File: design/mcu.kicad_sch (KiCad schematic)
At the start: 34 parts, among them J2 SWD_01X06, J3 DEBUG_SPI, U6 STM32H750VBTx, X1 ASTX-H11-25.000MHZ-T, X2 SIT8209AI-21-33S-100.000000X

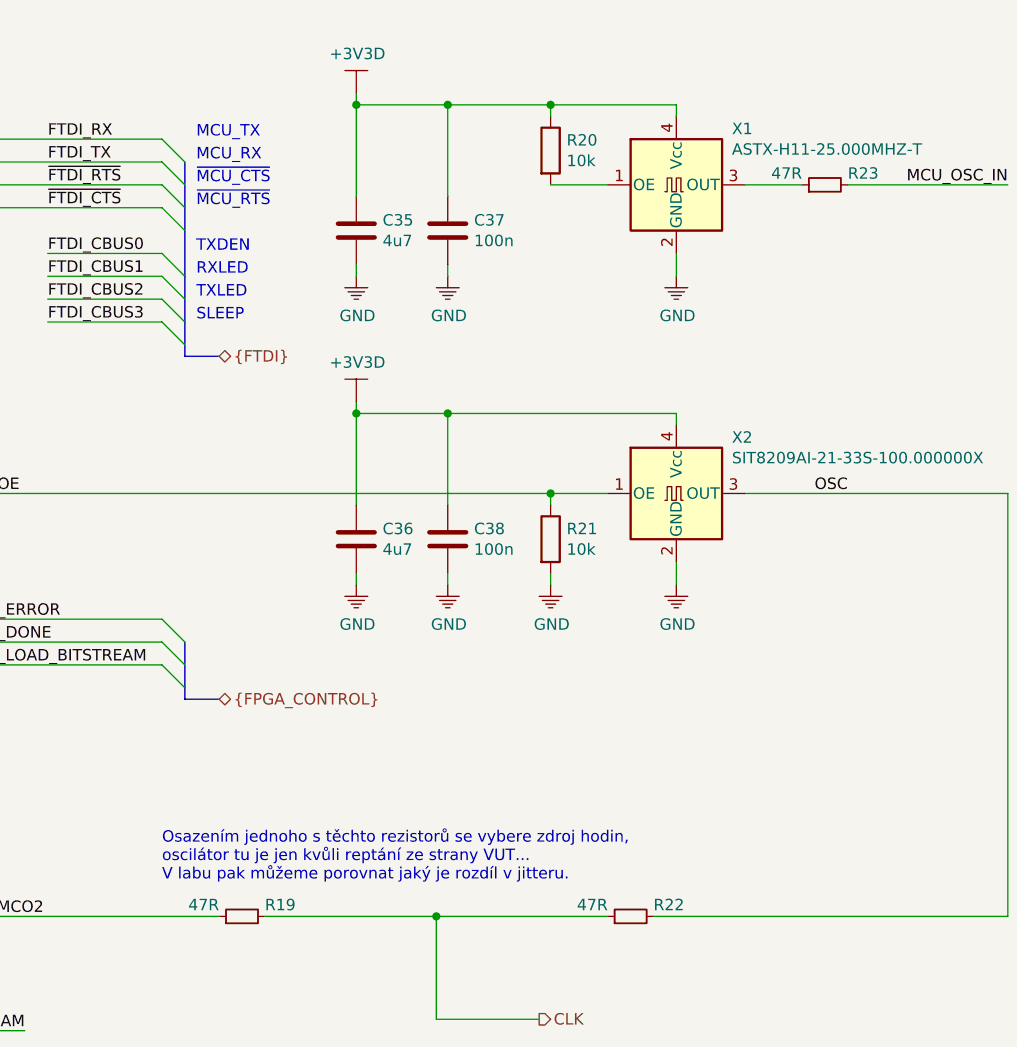
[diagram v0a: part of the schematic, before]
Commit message: Updated schematic
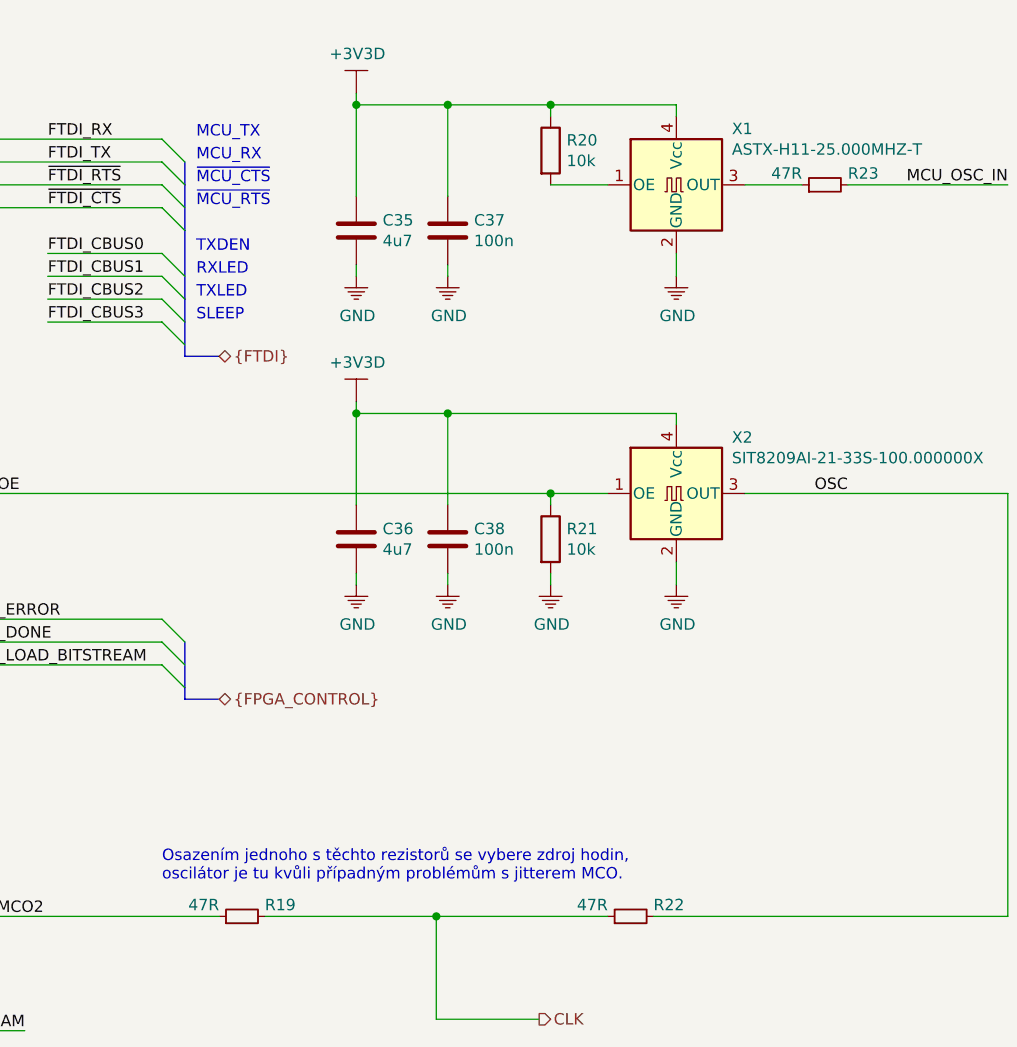
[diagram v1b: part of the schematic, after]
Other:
- note added: "Osazením jednoho s těchto rezistorů se vybere zdroj hodin, oscilátor je tu kvůli případným problémům s jitterem MCO."
- note removed: "Osazením jednoho s těchto rezistorů se vybere zdroj hodin, oscilátor tu je jen kvůli reptání ze strany VUT... V labu pak můžeme porovnat jaký je rozdíl v jitteru."
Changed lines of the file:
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@@
   (junction (at 236.22 25.4))
   (junction (at 262.89 26.67))
+  (no_connect (at 95.25 116.84))
+  (no_connect (at 140.97 48.26))
+  (no_connect (at 140.97 91.44))
+  (no_connect (at 95.25 152.4))
+  (no_connect (at 95.25 144.78))
+  (no_connect (at 140.97 96.52))
+  (no_connect (at 140.97 83.82))
+  (no_connect (at 140.97 58.42))
+  (no_connect (at 95.25 129.54))
+  (no_connect (at 140.97 93.98))
   (no_connect (at 140.97 43.18))
-  (no_connect (at 140.97 104.14))
+  (no_connect (at 95.25 132.08))
+  (no_connect (at 140.97 109.22))
+  (no_connect (at 140.97 134.62))
+  (no_connect (at 140.97 132.08))
+  (no_connect (at 140.97 129.54))
+  (no_connect (at 95.25 119.38))
+  (no_connect (at 140.97 119.38))
+  (no_connect (at 140.97 137.16))
+  (no_connect (at 140.97 101.6))
+  (no_connect (at 140.97 124.46))
+  (no_connect (at 95.25 137.16))
   (no_connect (at 140.97 149.86))
-  (no_connect (at 95.25 139.7))
+  (no_connect (at 140.97 45.72))
+  (no_connect (at 140.97 106.68))
+  (no_connect (at 140.97 53.34))
+  (no_connect (at 95.25 88.9))
+  (no_connect (at 95.25 109.22))
+  (no_connect (at 95.25 147.32))
+  (no_connect (at 140.97 76.2))
   (no_connect (at 95.25 99.06))
-  (no_connect (at 95.25 109.22))
-  (no_connect (at 140.97 134.62))
-  (no_connect (at 140.97 129.54))
+  (no_connect (at 140.97 50.8))
+  (no_connect (at 95.25 111.76))
+  (no_connect (at 95.25 76.2))
+  (no_connect (at 140.97 99.06))
   (no_connect (at 140.97 142.24))
   (no_connect (at 95.25 134.62))
+  (no_connect (at 95.25 104.14))
+  (no_connect (at 140.97 127))
   (no_connect (at 95.25 149.86))
-  (no_connect (at 140.97 93.98))
-  (no_connect (at 140.97 53.34))
-  (no_connect (at 140.97 137.16))
-  (no_connect (at 95.25 144.78))
-  (no_connect (at 140.97 76.2))
-  (no_connect (at 95.25 116.84))
-  (no_connect (at 140.97 91.44))
+  (no_connect (at 95.25 142.24))
+  (no_connect (at 95.25 83.82))
   (no_connect (at 140.97 38.1))
-  (no_connect (at 95.25 152.4))
-  (no_connect (at 95.25 119.38))
-  (no_connect (at 95.25 137.16))
-  (no_connect (at 140.97 99.06))
-  (no_connect (at 140.97 96.52))
-  (no_connect (at 140.97 124.46))
-  (no_connect (at 140.97 45.72))
-  (no_connect (at 140.97 132.08))
+  (no_connect (at 95.25 139.7))
+  (no_connect (at 140.97 157.48))
   (no_connect (at 95.25 81.28))
-  (no_connect (at 95.25 104.14))
-  (no_connect (at 95.25 83.82))
+  (no_connect (at 140.97 104.14))
+  (no_connect (at 140.97 144.78))
+  (no_connect (at 140.97 139.7))
+  (no_connect (at 140.97 162.56))
+  (no_connect (at 140.97 40.64))
+  (no_connect (at 95.25 114.3))
   (no_connect (at 140.97 55.88))
-  (no_connect (at 95.25 111.76))
-  (no_connect (at 140.97 127))
-  (no_connect (at 140.97 50.8))
-  (no_connect (at 140.97 157.48))
-  (no_connect (at 95.25 142.24))
-  (no_connect (at 95.25 76.2))
-  (no_connect (at 140.97 106.68))
-  (no_connect (at 140.97 48.26))
-  (no_connect (at 95.25 88.9))
-  (no_connect (at 140.97 40.64))
-  (no_connect (at 140.97 162.56))
-  (no_connect (at 140.97 109.22))
-  (no_connect (at 140.97 83.82))
-  (no_connect (at 95.25 147.32))
-  (no_connect (at 140.97 144.78))
-  (no_connect (at 140.97 101.6))
-  (no_connect (at 140.97 139.7))
-  (no_connect (at 95.25 114.3))
-  (no_connect (at 95.25 132.08))
-  (no_connect (at 140.97 119.38))
-  (no_connect (at 95.25 129.54))
-  (no_connect (at 140.97 58.42))
   (bus_entry (at 67.31 88.9) (size 2.54 -2.54))
   (bus_entry (at 67.31 93.98) (size 2.54 -2.54))
@@
   (bus (pts (xy 67.31 106.68) (xy 67.31 111.76)))
   (bus (pts (xy 67.31 111.76) (xy 67.31 113.03)))
-  (bus (pts (xy 182.88 63.5) (xy 182.88 68.58)))
-  (bus (pts (xy 182.88 68.58) (xy 182.88 76.2)))
-  (bus (pts (xy 182.88 76.2) (xy 182.88 81.28)))
+  (bus (pts (xy 182.88 63.5) (xy 182.88 66.04)))
+  (bus (pts (xy 182.88 66.04) (xy 182.88 71.12)))
+  (bus (pts (xy 182.88 71.12) (xy 182.88 78.74)))
+  (bus (pts (xy 182.88 78.74) (xy 182.88 81.28)))
   (bus (pts (xy 182.88 81.28) (xy 182.88 85.09)))
   (bus (pts (xy 182.88 85.09) (xy 186.69 85.09)))
@@
   (polyline (pts (xy 283.21 13.97) (xy 283.21 44.45)))
   (polyline (pts (xy 283.21 44.45) (xy 259.08 44.45)))
-  (text "Osazením jednoho s těchto rezistorů se vybere zdroj hodin,\noscilátor tu je jen kvůli reptání ze strany VUT...\nV labu pak můžeme porovnat jaký je rozdíl v jitteru."
+  (text "Osazením jednoho s těchto rezistorů se vybere zdroj hodin,\noscilátor je tu kvůli případným problémům s jitterem MCO."
     (at 180.34 143.51 0)
     (effects (font (size 1.27 1.27)) (justify left bottom))

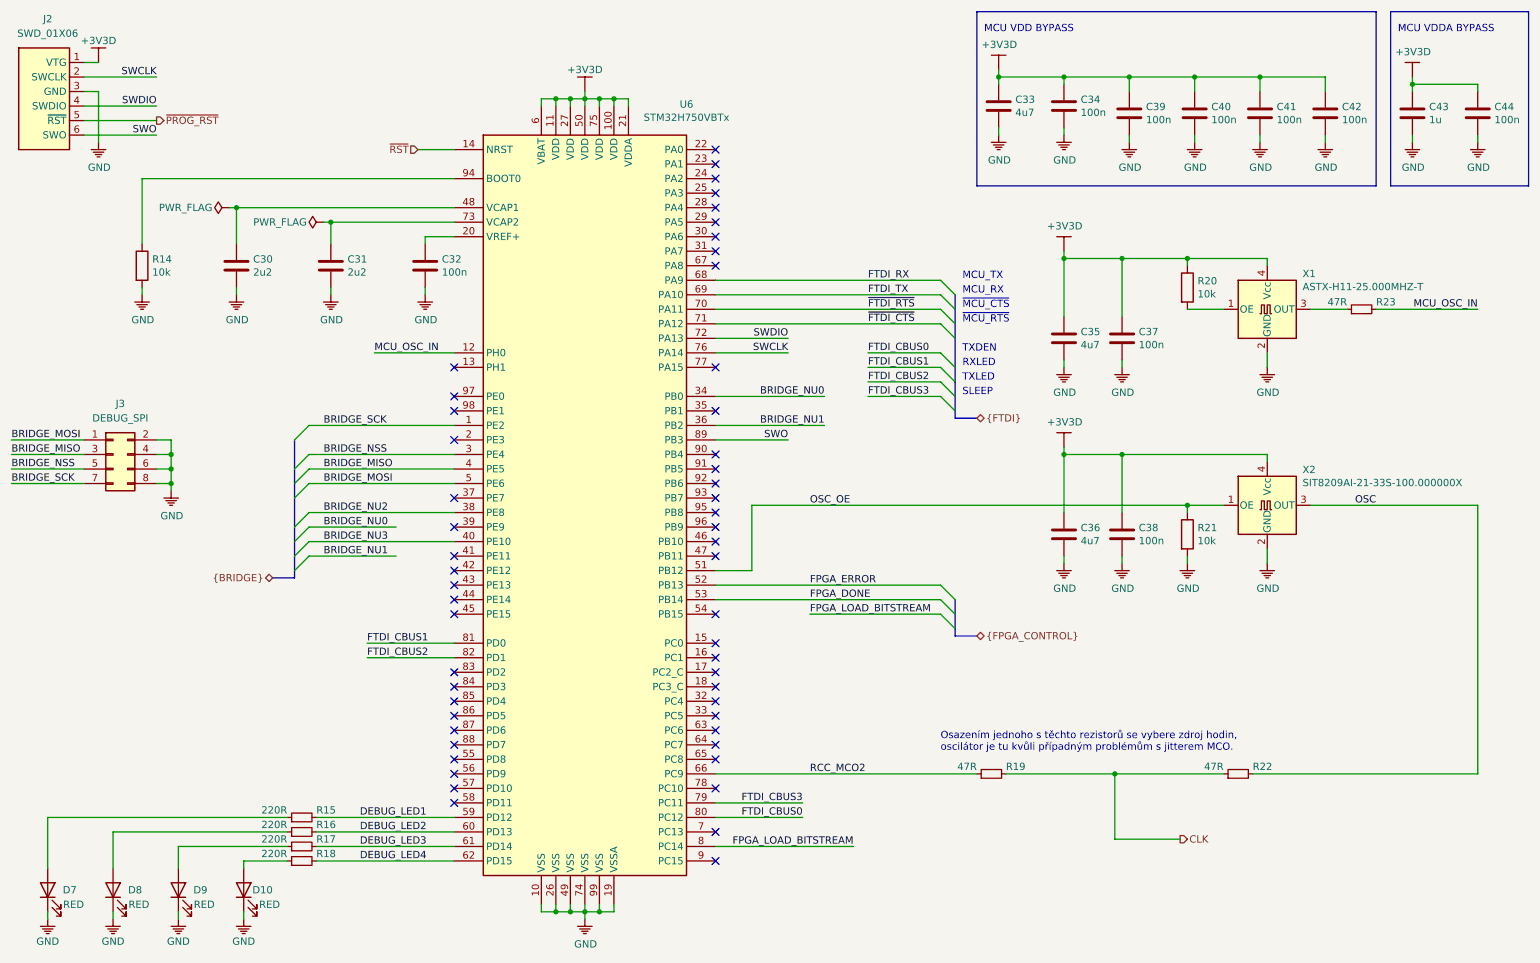
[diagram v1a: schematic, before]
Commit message: Updated LNA
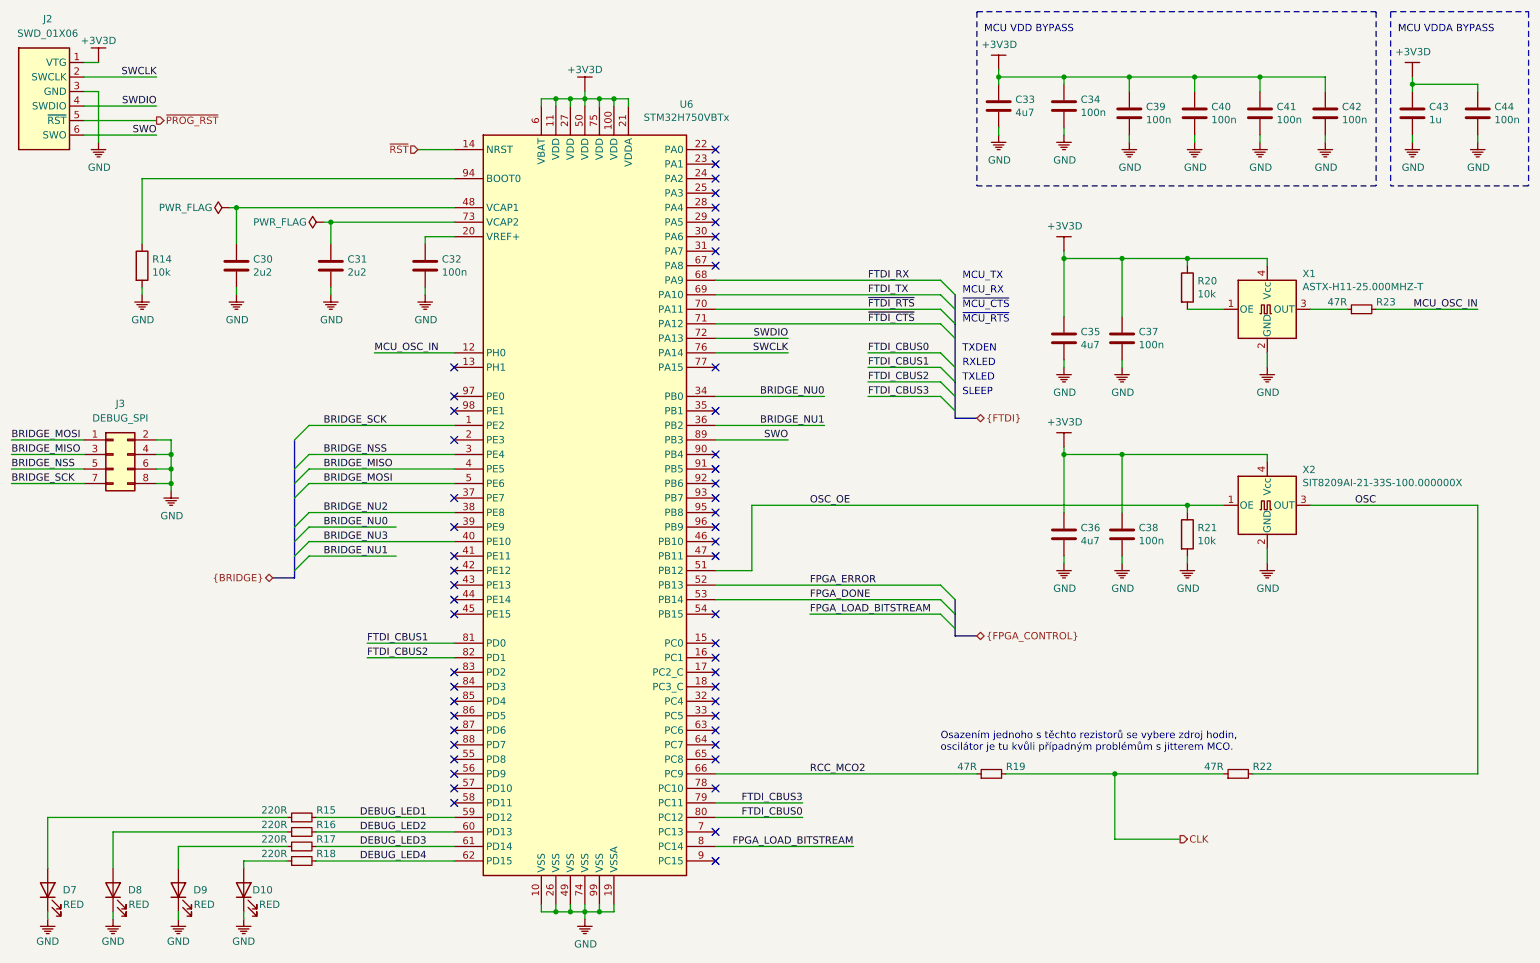
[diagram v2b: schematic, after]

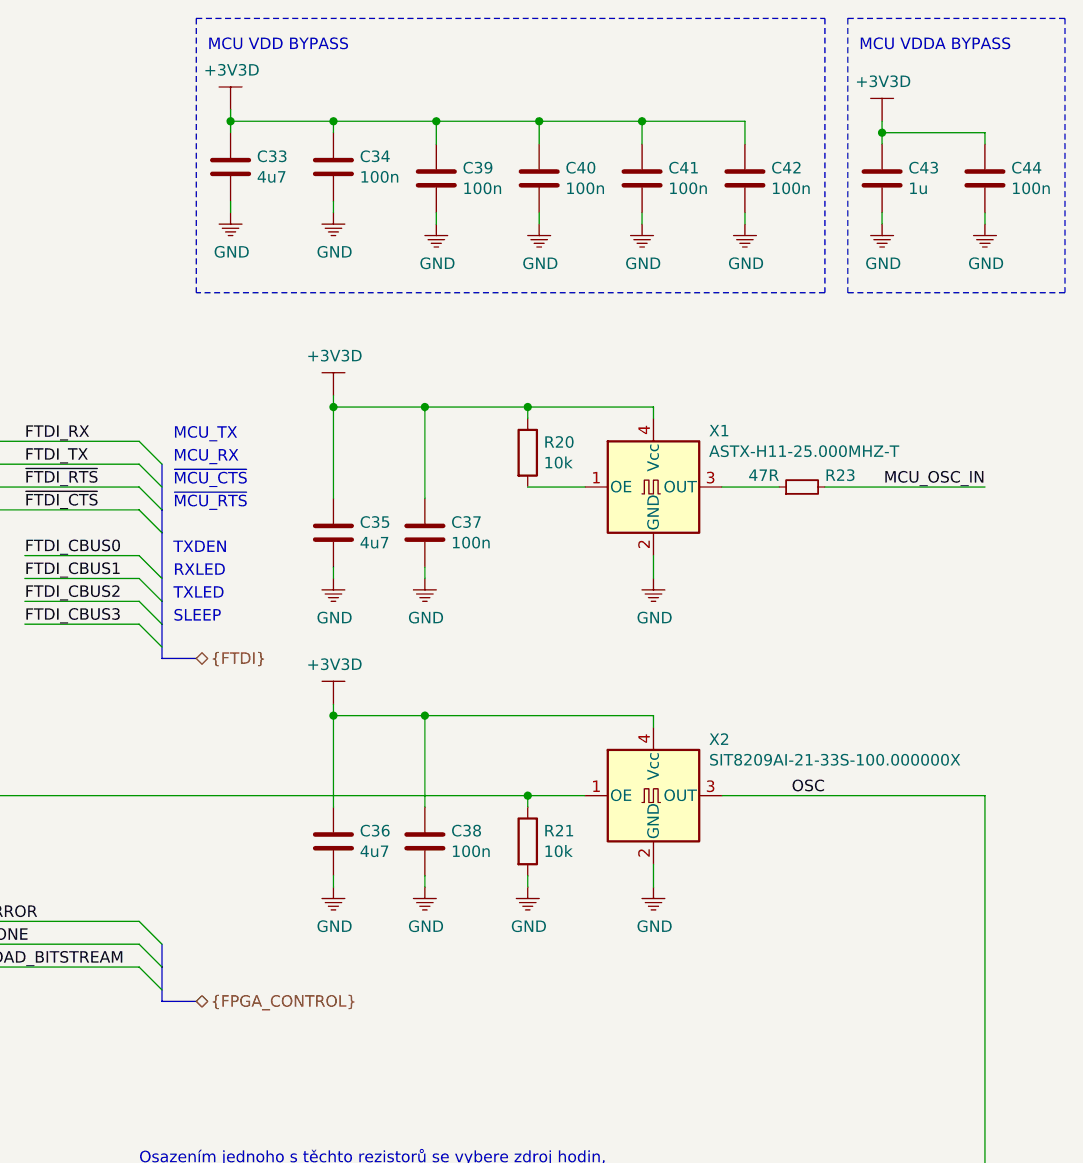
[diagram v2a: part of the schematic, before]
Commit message: Updated notes
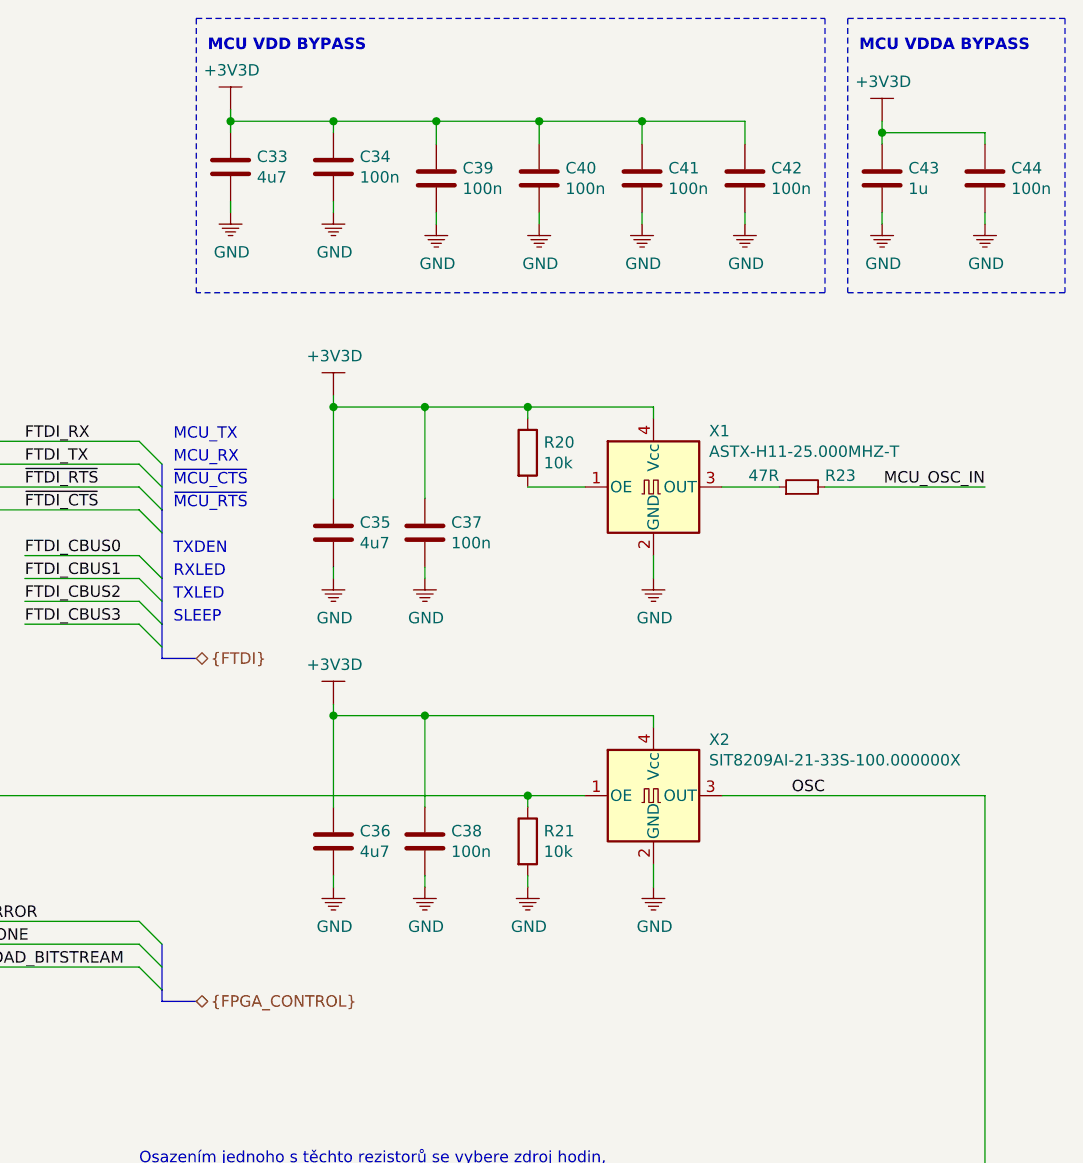
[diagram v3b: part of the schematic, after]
